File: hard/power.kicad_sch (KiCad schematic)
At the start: 45 parts, among them J3 Vin, J4 USB_B_Mini, J5 Vout 5V, Q4 IRLML9301, SW7 Power_button, U5 XC6705A331MR-G, U6 TPS563201

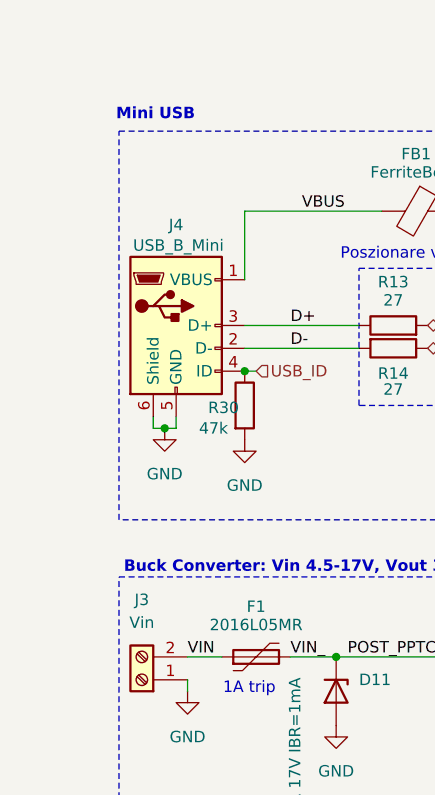
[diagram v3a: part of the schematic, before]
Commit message: update
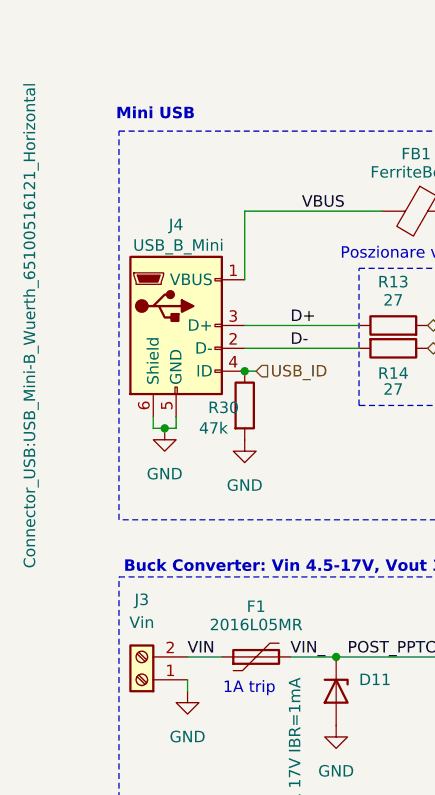
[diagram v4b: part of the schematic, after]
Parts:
- C30, C31, C32, C33, C34, C35, C36, C37, C38, C39, C40: footprint (none) -> Capacitor_Tantalum_SMD:CP_EIA-1608-08_AVX-J
- D11, D12: footprint (none) -> Diode_SMD:D_SMA
- D13, D14, D19: footprint (none) -> Diode_SMD:D_SOD-123
- D15: footprint (none) -> Diode_SMD:D_SOD-123F
- D16: footprint (none) -> LED_SMD:LED_0805_2012Metric
- D17: footprint (none) -> Diode_SMD:D_SOD-323_HandSoldering
- D18: footprint (none) -> LED_SMD:LED_0805_2012Metric_Pad1.15x1.40mm_HandSolder
- F1: footprint (none) -> Fuse:Fuse_1206_3216Metric
- FB1: footprint (none) -> Capacitor_SMD:C_0805_2012Metric
- J4: footprint (none) -> Connector_USB:USB_Mini-B_Wuerth_65100516121_Horizontal
- L1: footprint (none) -> Capacitor_SMD:C_0603_1608Metric
- R13, R14, R15, R16, R17, R18, R19, R20, R21, R22, R23, R29, R30: footprint (none) -> Resistor_SMD:R_0201_0603Metric
- SW7: footprint (none) -> Button_Switch_SMD:Nidec_Copal_CAS-120A
- TP4: footprint (none) -> TestPoint:TestPoint_THTPad_D1.5mm_Drill0.7mm
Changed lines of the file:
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@@
 		)
 		(property "Netclass" "TP2"
-			(at 112.776 22.098 0)
+			(at 112.522 21.59 0)
 			(effects
 				(font
@@
 			)
 		)
-		(property "Footprint" ""
+		(property "Footprint" "Diode_SMD:D_SOD-123"
 			(at 77.47 25.4 90)
 			(effects
@@
 			)
 		)
-		(property "Footprint" ""
+		(property "Footprint" "Capacitor_Tantalum_SMD:CP_EIA-1608-08_AVX-J"
 			(at 180.0352 82.55 0)
 			(effects
@@
 			)
 		)
-		(property "Footprint" ""
+		(property "Footprint" "Resistor_SMD:R_0201_0603Metric"
 			(at 94.742 83.82 90)
 			(effects
@@
 			)
 		)
-		(property "Footprint" ""
+		(property "Footprint" "Resistor_SMD:R_0201_0603Metric"
 			(at 45.72 38.862 90)
 			(effects
@@
 			)
 		)
-		(property "Footprint" ""
+		(property "Footprint" "Capacitor_Tantalum_SMD:CP_EIA-1608-08_AVX-J"
 			(at 59.3852 82.55 0)
 			(effects
@@
 			)
 		)
-		(property "Footprint" ""
+		(property "Footprint" "LED_SMD:LED_0805_2012Metric"
 			(at 158.75 31.75 0)
 			(effects
@@
 			)
 		)
-		(property "Footprint" ""
-			(at 25.4 39.37 0)
+		(property "Footprint" "Connector_USB:USB_Mini-B_Wuerth_65100516121_Horizontal"
+			(at 5.334 38.1 90)
 			(effects
 				(font
 					(size 1.27 1.27)
 				)
-				(hide yes)
 			)
 		)
@@
 			)
 		)
-		(property "Footprint" ""
+		(property "Footprint" "TestPoint:TestPoint_THTPad_D1.5mm_Drill0.7mm"
 			(at 196.85 40.64 0)
 			(effects
@@
 			)
 		)
-		(property "Footprint" ""
+		(property "Footprint" "Capacitor_SMD:C_0805_2012Metric"
 			(at 48.26 23.622 90)
 			(effects
@@
 			)
 		)
-		(property "Footprint" ""
+		(property "Footprint" "Diode_SMD:D_SMA"
 			(at 54.61 74.93 0)
 			(effects
@@
 			)
 		)
-		(property "Footprint" ""
+		(property "Footprint" "Resistor_SMD:R_0201_0603Metric"
 			(at 27.432 46.99 90)
 			(effects
@@
 			)
 		)
-		(property "Footprint" ""
+		(property "Footprint" "Resistor_SMD:R_0201_0603Metric"
 			(at 241.3 37.338 90)
 			(effects
@@
 			)
 		)
-		(property "Footprint" ""
+		(property "Footprint" "Resistor_SMD:R_0201_0603Metric"
 			(at 189.992 86.36 90)
 			(effects
@@
 			)
 		)
-		(property "Footprint" ""
+		(property "Footprint" "Capacitor_Tantalum_SMD:CP_EIA-1608-08_AVX-J"
 			(at 69.5452 82.55 0)
 			(effects
@@
 			)
 		)
-		(property "Footprint" ""
+		(property "Footprint" "LED_SMD:LED_0805_2012Metric_Pad1.15x1.40mm_HandSolder"
 			(at 191.77 78.74 0)
 			(effects
@@
 			)
 		)
-		(property "Footprint" ""
+		(property "Footprint" "Resistor_SMD:R_0201_0603Metric"
 			(at 45.72 39.878 90)
 			(effects
@@
 			)
 		)
-		(property "Footprint" ""
+		(property "Footprint" "Button_Switch_SMD:Nidec_Copal_CAS-120A"
 			(at 81.28 109.22 0)
 			(effects
@@
 			)
 		)
-		(property "Footprint" ""
+		(property "Footprint" "Resistor_SMD:R_0201_0603Metric"
 			(at 234.442 31.75 90)
 			(effects
@@
 			)
 		)
-		(property "Footprint" ""
+		(property "Footprint" "Capacitor_Tantalum_SMD:CP_EIA-1608-08_AVX-J"
 			(at 111.4552 35.56 0)
 			(effects
@@
 			)
 		)
-		(property "Footprint" ""
+		(property "Footprint" "Capacitor_Tantalum_SMD:CP_EIA-1608-08_AVX-J"
 			(at 136.1948 74.93 0)
 			(effects
@@
 			)
 		)
-		(property "Footprint" ""
+		(property "Footprint" "Diode_SMD:D_SOD-323_HandSoldering"
 			(at 256.54 39.37 0)
 			(effects
@@
 			)
 		)
-		(property "Footprint" ""
+		(property "Footprint" "Diode_SMD:D_SOD-123"
 			(at 87.63 93.98 0)
 			(effects
@@
 			)
 		)
-		(property "Footprint" ""
+		(property "Footprint" "Capacitor_Tantalum_SMD:CP_EIA-1608-08_AVX-J"
 			(at 177.4952 43.18 0)
 			(effects
@@
 			)
 		)
-		(property "Footprint" ""
+		(property "Footprint" "Diode_SMD:D_SOD-123"
 			(at 210.82 74.93 90)
 			(effects
@@
 			)
 		)
-		(property "Footprint" ""
+		(property "Footprint" "Capacitor_Tantalum_SMD:CP_EIA-1608-08_AVX-J"
 			(at 144.4752 35.56 0)
 			(effects
@@
 			)
 		)
-		(property "Footprint" ""
+		(property "Footprint" "Resistor_SMD:R_0201_0603Metric"
 			(at 82.55 46.228 90)
 			(effects
@@
 			)
 		)
-		(property "Footprint" ""
+		(property "Footprint" "Capacitor_Tantalum_SMD:CP_EIA-1608-08_AVX-J"
 			(at 169.8752 82.55 0)
 			(effects
@@
 			)
 		)
-		(property "Footprint" ""
+		(property "Footprint" "Fuse:Fuse_1206_3216Metric"
 			(at 35.56 73.66 0)
 			(effects
@@
 			)
 		)
-		(property "Footprint" ""
+		(property "Footprint" "Capacitor_SMD:C_0603_1608Metric"
 			(at 143.51 74.93 0)
 			(effects
@@
 			)
 		)
-		(property "Footprint" ""
+		(property "Footprint" "Resistor_SMD:R_0201_0603Metric"
 			(at 156.972 39.37 90)
 			(effects
@@
 			)
 		)
-		(property "Footprint" ""
+		(property "Footprint" "Capacitor_Tantalum_SMD:CP_EIA-1608-08_AVX-J"
 			(at 80.9752 82.55 0)
 			(effects
@@
 			)
 		)
-		(property "Footprint" ""
+		(property "Footprint" "Resistor_SMD:R_0201_0603Metric"
 			(at 174.752 31.75 90)
 			(effects
@@
 			)
 		)
-		(property "Footprint" ""
+		(property "Footprint" "Resistor_SMD:R_0201_0603Metric"
 			(at 146.812 88.9 90)
 			(effects
@@
 			)
 		)
-		(property "Footprint" ""
+		(property "Footprint" "Diode_SMD:D_SMA"
 			(at 39.37 78.74 0)
 			(effects
@@
 			)
 		)
-		(property "Footprint" ""
+		(property "Footprint" "Diode_SMD:D_SOD-123F"
 			(at 87.63 104.14 0)
 			(effects
@@
 			)
 		)
-		(property "Footprint" ""
+		(property "Footprint" "Capacitor_Tantalum_SMD:CP_EIA-1608-08_AVX-J"
 			(at 160.9852 82.55 0)
 			(effects
@@
 			)
 		)
-		(property "Footprint" ""
+		(property "Footprint" "Capacitor_Tantalum_SMD:CP_EIA-1608-08_AVX-J"
 			(at 246.0752 43.18 0)
 			(effects
@@
 			)
 		)
-		(property "Footprint" ""
+		(property "Footprint" "Resistor_SMD:R_0201_0603Metric"
 			(at 234.442 39.37 90)
 			(effects
@@
 			)
 		)
-		(property "Footprint" ""
+		(property "Footprint" "Resistor_SMD:R_0201_0603Metric"
 			(at 146.812 78.74 90)
 			(effects

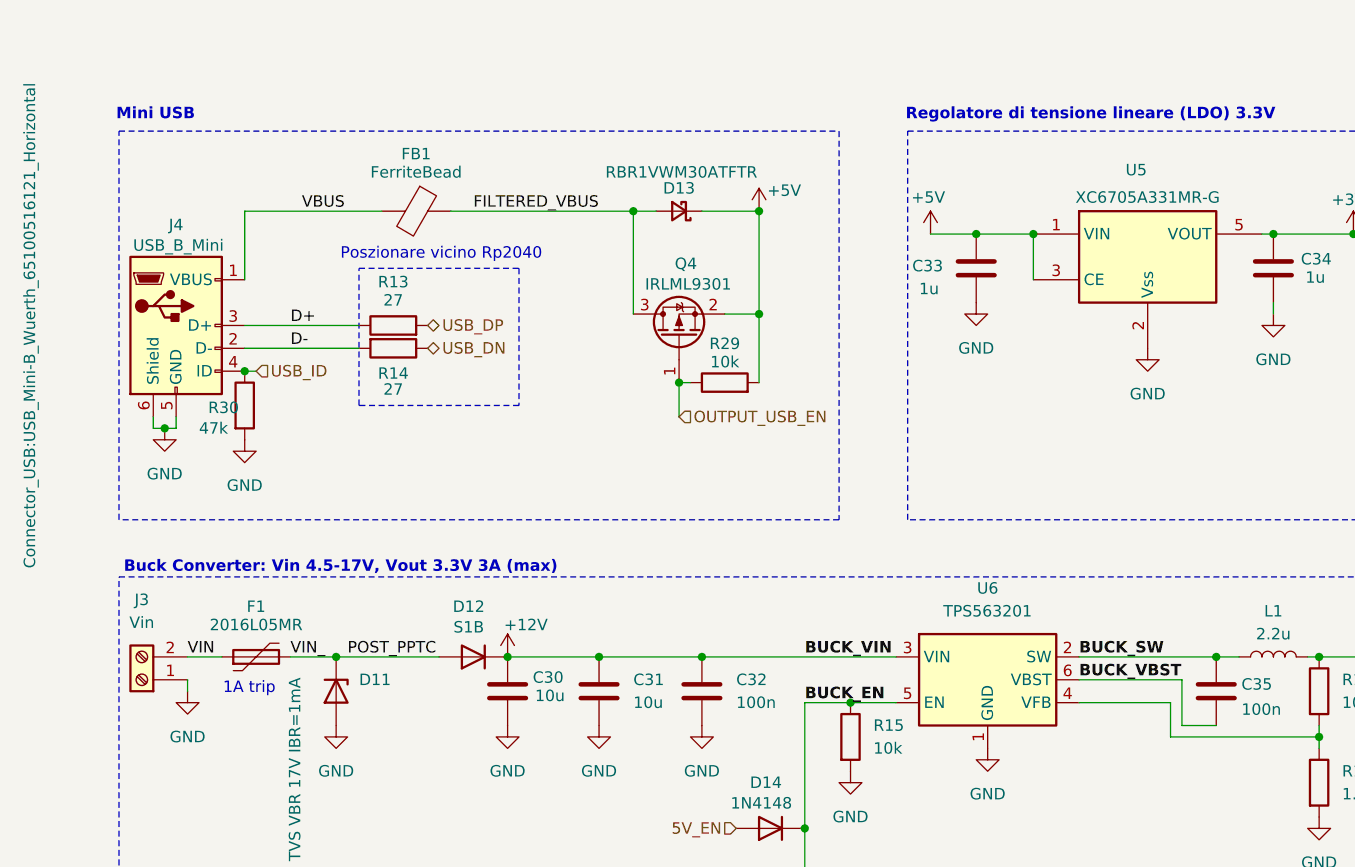
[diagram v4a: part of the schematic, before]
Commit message: update
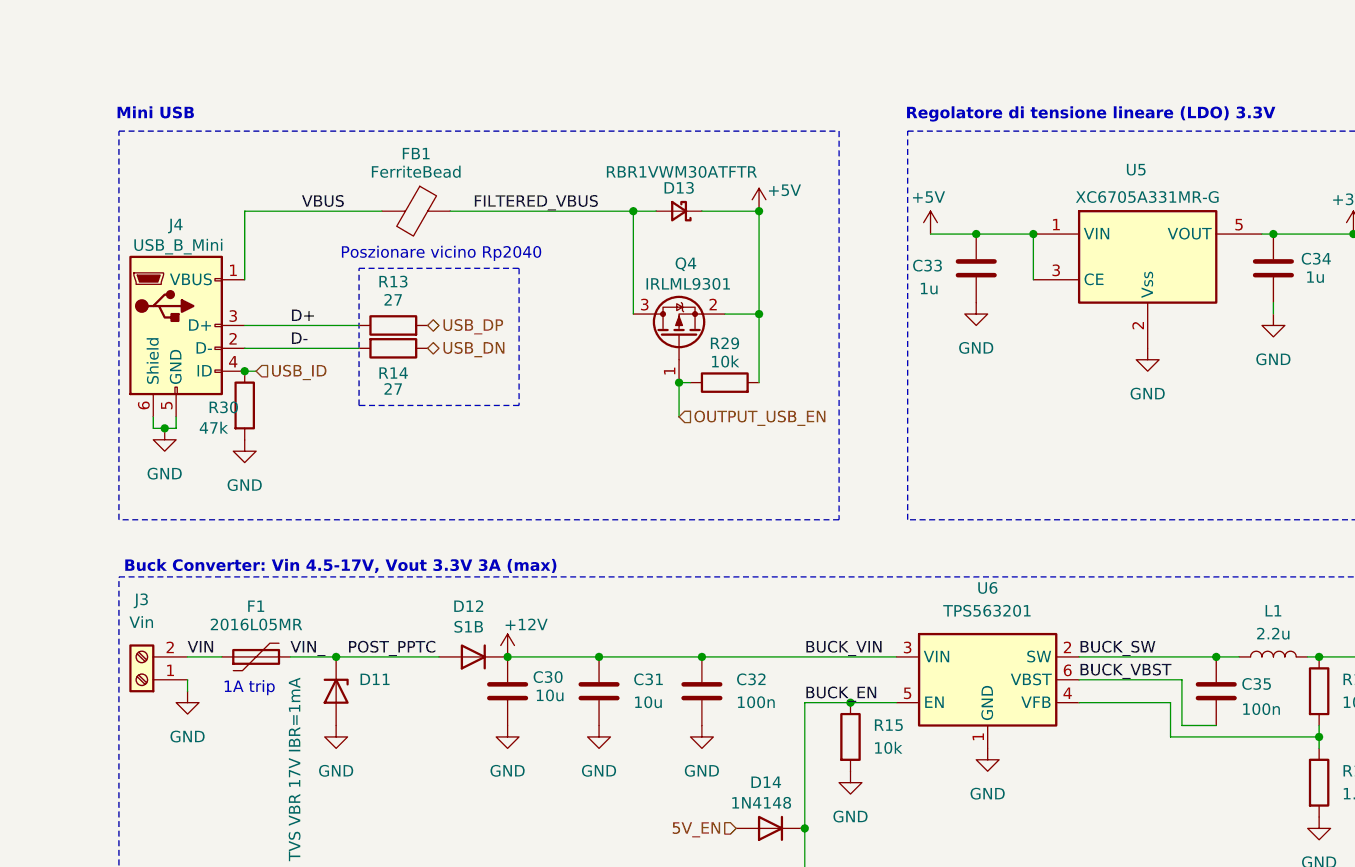
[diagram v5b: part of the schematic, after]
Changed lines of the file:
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@@
 			(font
 				(size 1.27 1.27)
-				(thickness 0.254)
-				(bold yes)
+				(thickness 0.1588)
 			)
 			(justify left bottom)
@@
 			(font
 				(size 1.27 1.27)
-				(thickness 0.254)
-				(bold yes)
+				(thickness 0.1588)
 			)
 			(justify left bottom)
@@
 			(font
 				(size 1.27 1.27)
-				(thickness 0.254)
-				(bold yes)
+				(thickness 0.1588)
 			)
 			(justify left bottom)
@@
 			(font
 				(size 1.27 1.27)
-				(thickness 0.254)
-				(bold yes)
+				(thickness 0.1588)
 			)
 			(justify left bottom)
@@
 		(shape round)
 		(at 29.21 25.4 0)
+		(fields_autoplaced yes)
 		(effects
 			(font
@@
 		)
 		(property "Netclass" "TP1"
-			(at 26.924 18.542 0)
+			(at 29.9085 22.86 0)
 			(effects
 				(font
@@
 		)
 		(property "Component Class" "VBUS"
-			(at 26.416 21.082 0)
+			(at 29.9085 24.3205 0)
 			(effects
 				(font
@@
 					(size 1.27 1.27)
 				)
-			)
-		)
+				(hide yes)
+			)
+		)

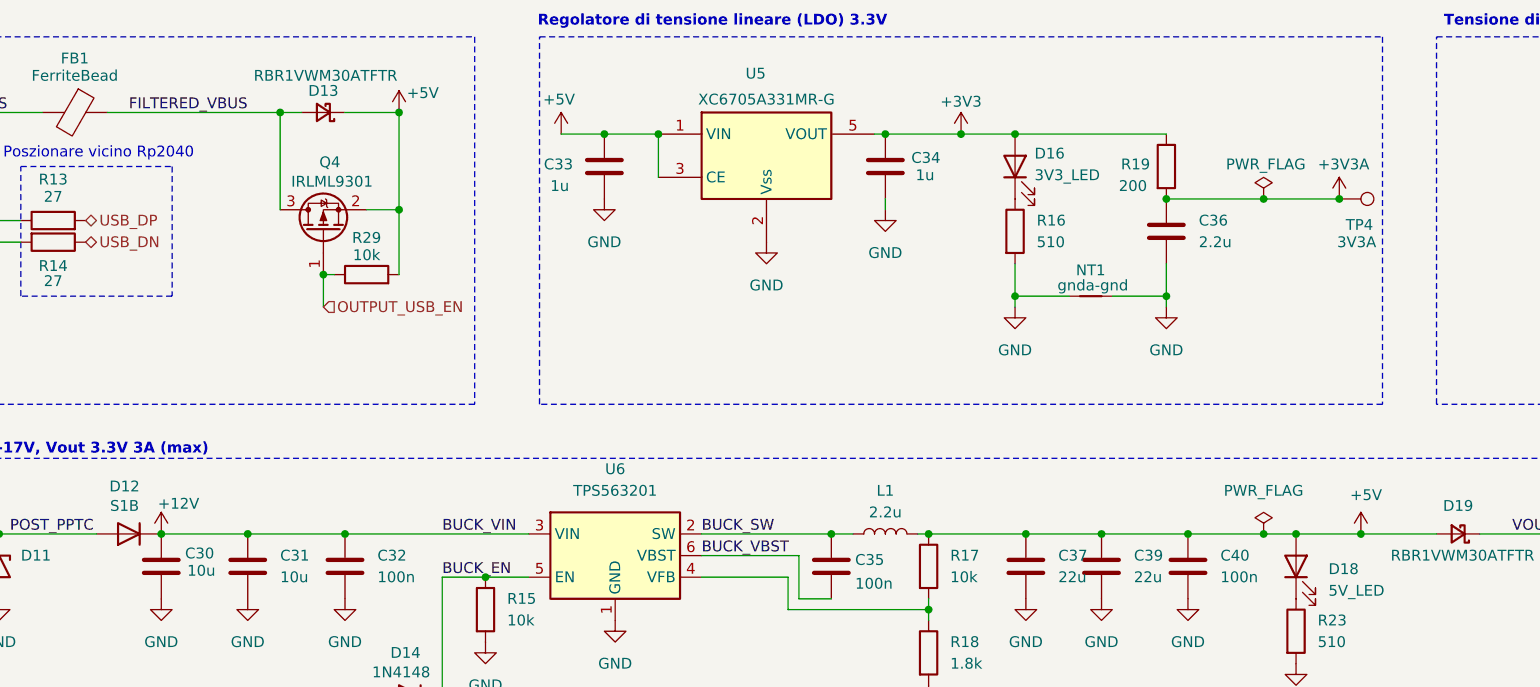
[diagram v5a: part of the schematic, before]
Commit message: update
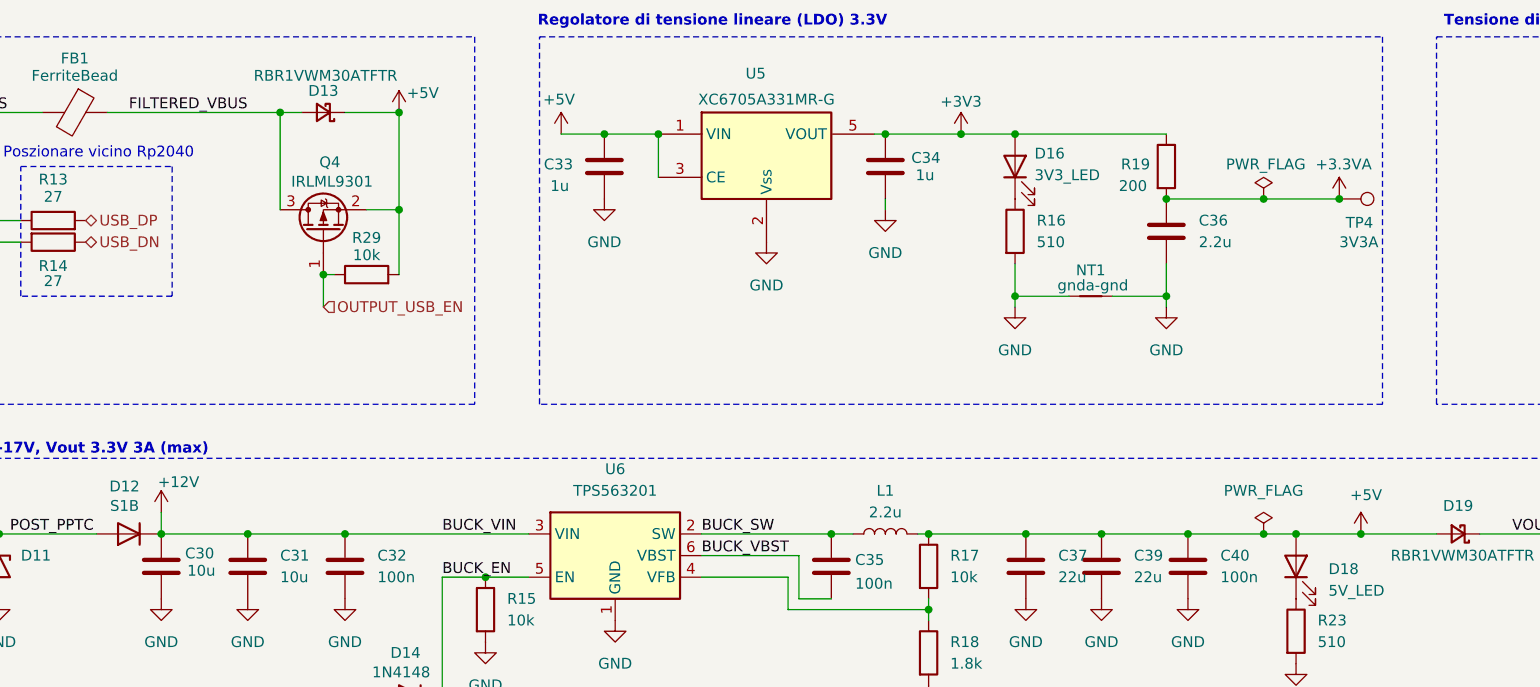
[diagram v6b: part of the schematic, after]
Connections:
- net +3V3A renamed +3.3VA
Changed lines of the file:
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@@
 	(wire
 		(pts
+			(xy 58.42 72.39) (xy 58.42 74.93)
+		)
+		(stroke
+			(width 0)
+			(type default)
+		)
+	)
+	(wire
+		(pts
 			(xy 121.92 77.47) (xy 133.35 77.47)
 		)
@@
 			(justify left bottom)
 		)
-		(property "Netclass" "TP2"
+		(property "Netclass" "5V"
 			(at 112.522 21.59 0)
 			(effects
@@
 			)
 		)
-		(property "Component Class" "5V"
+		(property "Component Class" "TP2"
 			(at 113.03 23.876 0)
 			(effects
@@
 		(shape round)
 		(at 29.21 25.4 0)
-		(fields_autoplaced yes)
 		(effects
 			(font
@@
 			(justify left bottom)
 		)
-		(property "Netclass" "TP1"
-			(at 29.9085 22.86 0)
+		(property "Netclass" "VBUS"
+			(at 29.972 20.828 0)
 			(effects
 				(font
@@
 			)
 		)
-		(property "Component Class" "VBUS"
-			(at 29.9085 24.3205 0)
+		(property "Component Class" "TP1"
+			(at 29.972 23.876 0)
 			(effects
 				(font
@@
 	)
 	(symbol
+		(lib_name "VD_1")
 		(lib_id "power:VD")
 		(at 196.85 35.56 0)
@@
 			)
 		)
-		(property "Value" "+3V3A"
+		(property "Value" "+3.3VA"
 			(at 197.358 31.496 0)
 			(effects
@@
 		(dnp no)
 		(property "Reference" "TP4"
-			(at 197.612 38.608 90)
+			(at 197.612 38.354 90)
 			(effects
 				(font
@@
 		)
 		(property "Value" "3V3A"
-			(at 196.596 40.64 90)
+			(at 196.85 40.64 90)
 			(effects
 				(font
@@
 	)
 	(symbol
+		(lib_name "PWR_FLAG_1")
 		(lib_id "power:PWR_FLAG")
 		(at 187.96 35.56 0)
@@
 	(symbol
 		(lib_id "power:VCC")
-		(at 58.42 74.93 0)
+		(at 58.42 72.39 0)
 		(unit 1)
 		(exclude_from_sim no)
@@
 		(dnp no)
 		(property "Reference" "#PWR048"
-			(at 58.42 78.74 0)
+			(at 58.42 76.2 0)
 			(effects
 				(font
@@
 		)
 		(property "Value" "+12V"
-			(at 60.452 71.374 0)
+			(at 60.452 68.834 0)
 			(effects
 				(font
@@
 		)
 		(property "Footprint" ""
-			(at 58.42 74.93 0)
+			(at 58.42 72.39 0)
 			(effects
 				(font
@@
 		)
 		(property "Datasheet" ""
-			(at 58.42 74.93 0)
+			(at 58.42 72.39 0)
 			(effects
 				(font
@@
 		)
 		(property "Description" "Power symbol creates a global label with name \"VCC\""
-			(at 58.42 74.93 0)
+			(at 58.42 72.39 0)
 			(effects
 				(font
